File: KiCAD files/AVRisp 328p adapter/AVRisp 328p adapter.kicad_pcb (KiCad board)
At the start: 2 copper layers, 38.1 x 38.1 mm, 4 parts, among them J1 Conn_01x01_Male, J2 Conn_01x02_Male, J3 Conn_01x06_Male, J4 ISP

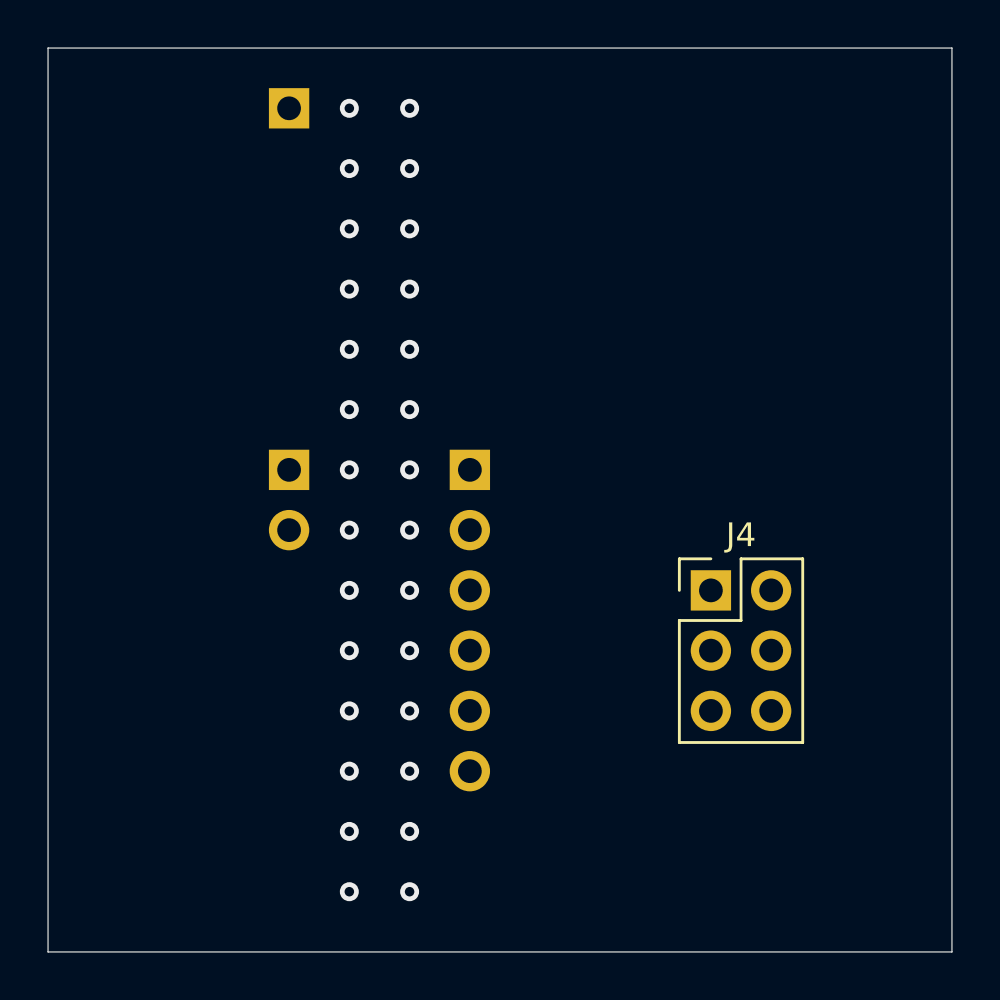
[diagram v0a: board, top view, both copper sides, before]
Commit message: office
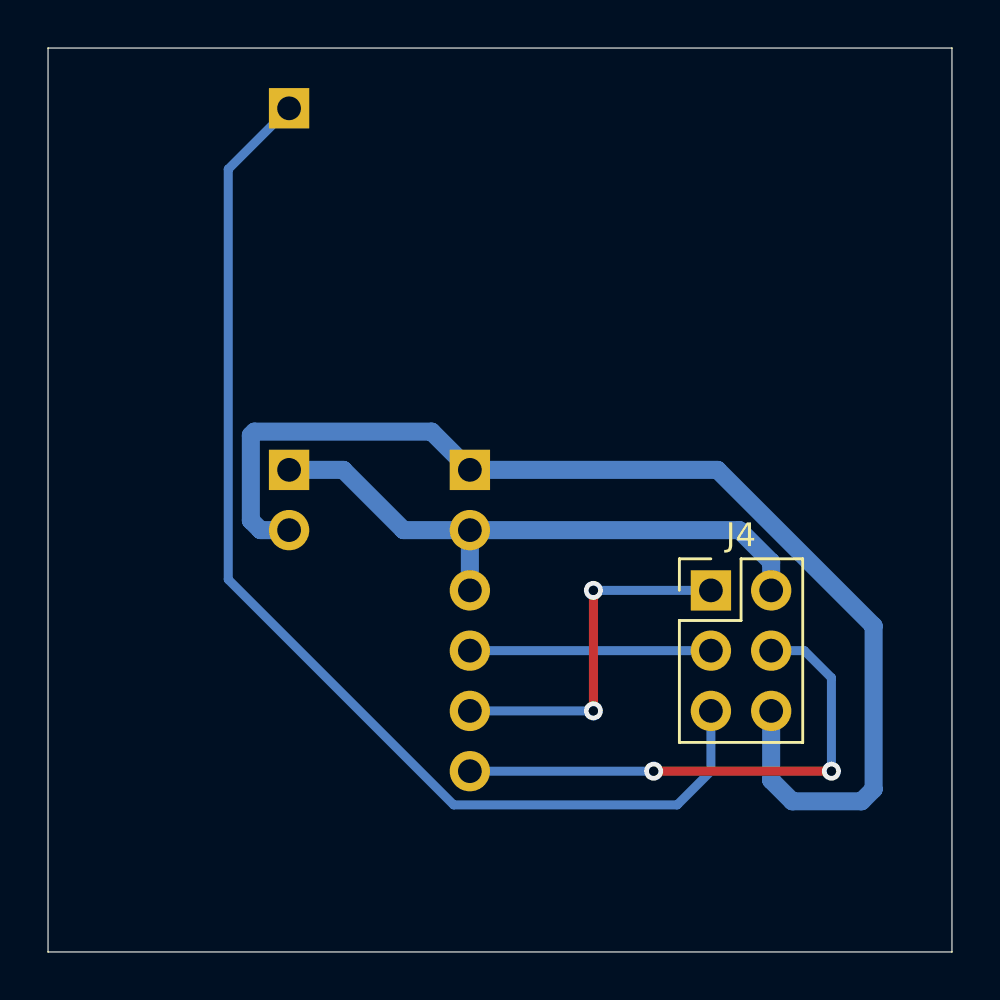
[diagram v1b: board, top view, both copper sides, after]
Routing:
- net GND: track 0.00 -> 49.8 mm
- net /RESET: track 0.00 -> 48.3 mm
- net +5V: track 0.00 -> 25.7 mm
- net /MOSI: track 0.00 -> 22.2 mm, vias 0 -> 2
- net /MISO: track 0.00 -> 15.2 mm, vias 0 -> 2
- net /SCK: track 0.00 -> 10.2 mm
- net (no net): vias 28 -> 0
